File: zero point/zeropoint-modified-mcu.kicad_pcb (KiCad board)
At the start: 2 copper layers, 121.4 x 77.7 mm, 29 parts, among them J1 TrackPoint, SW20 SW_PUSH

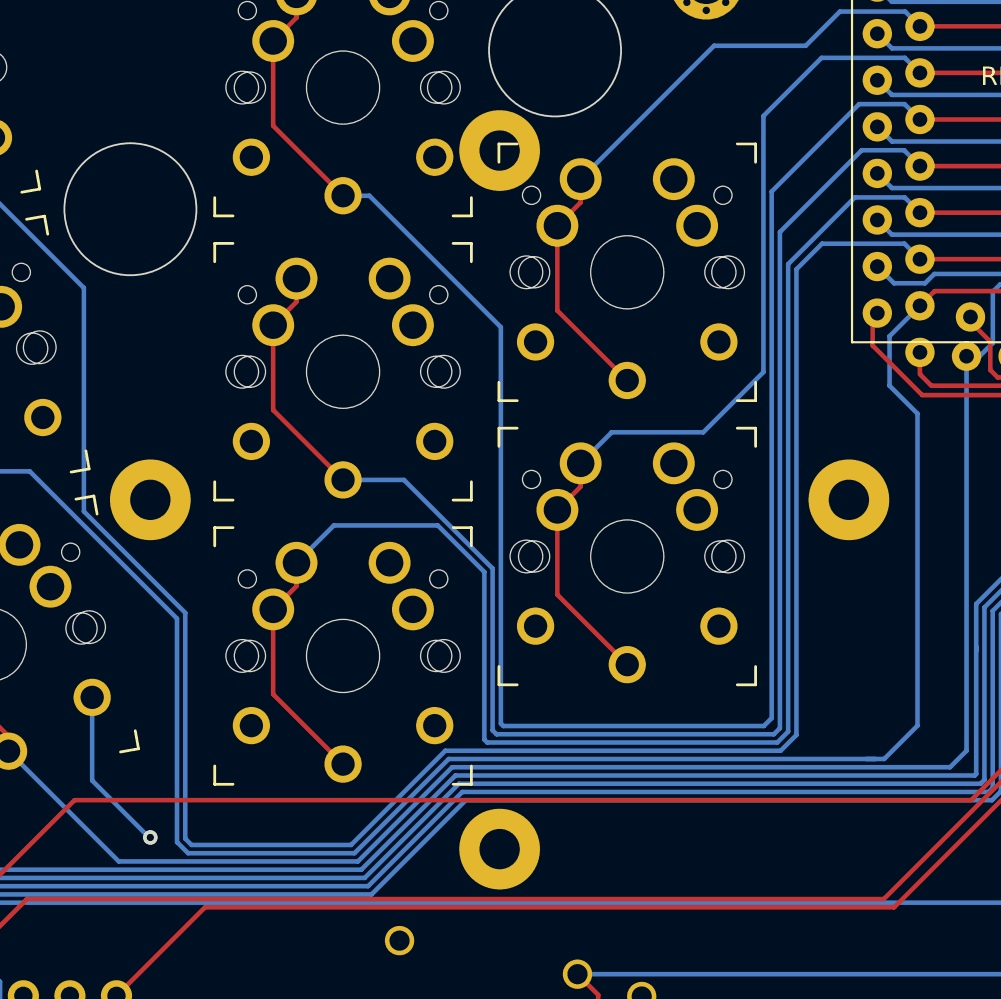
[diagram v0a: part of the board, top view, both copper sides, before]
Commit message: move tentig puck a little
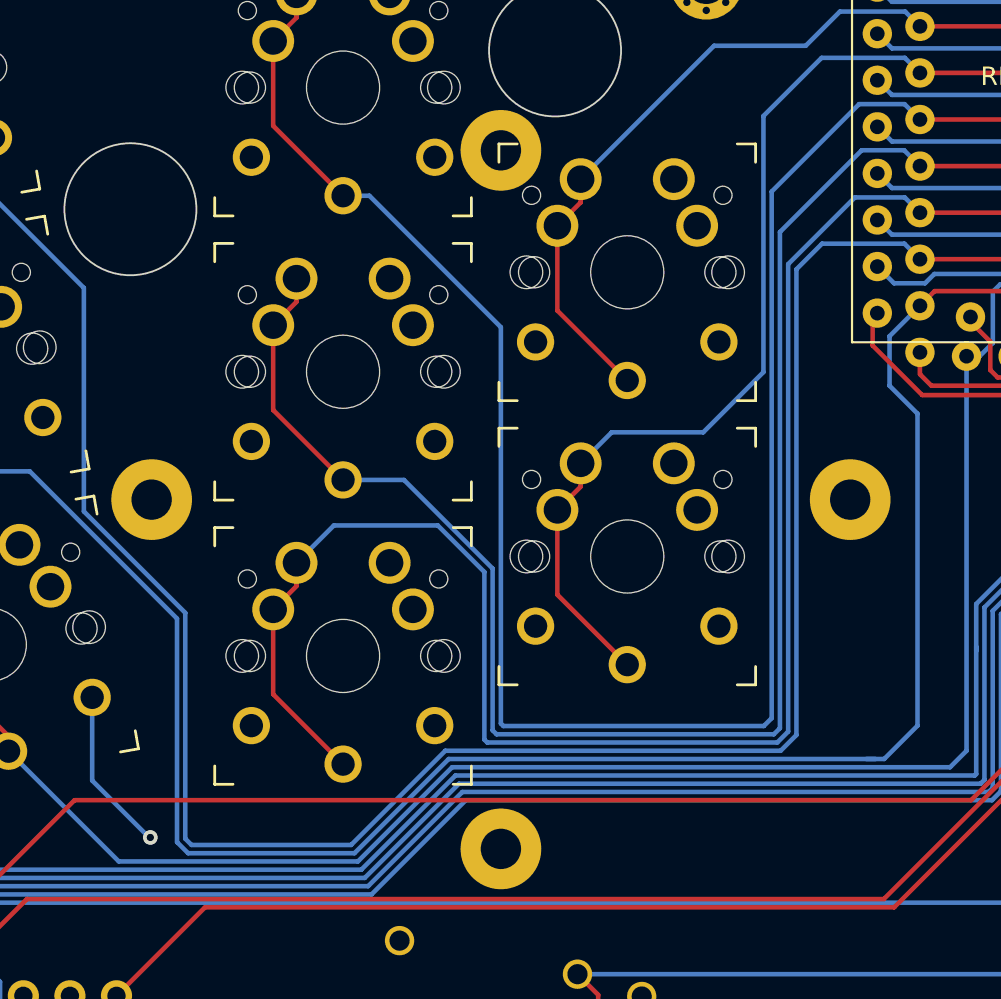
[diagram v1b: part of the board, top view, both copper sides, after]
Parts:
- moved REF** 0.07 mm to (219.3, 151.2)
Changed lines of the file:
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@@
   )
   (footprint "kbd:Tenting_Puck2" (layer "F.Cu")
-    (at 219.270692 151.256844)
+    (at 219.342045 151.245714)
     (attr through_hole)
     (fp_text reference "REF**" (at 7.6835 1.4605) (layer "F.Fab")
